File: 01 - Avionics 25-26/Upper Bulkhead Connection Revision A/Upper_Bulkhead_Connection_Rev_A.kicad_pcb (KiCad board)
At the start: 2 copper layers, 38 x 40.9 mm, 4 parts, among them J1 2601-3108, J2 M12A-08PMMP-SF8001

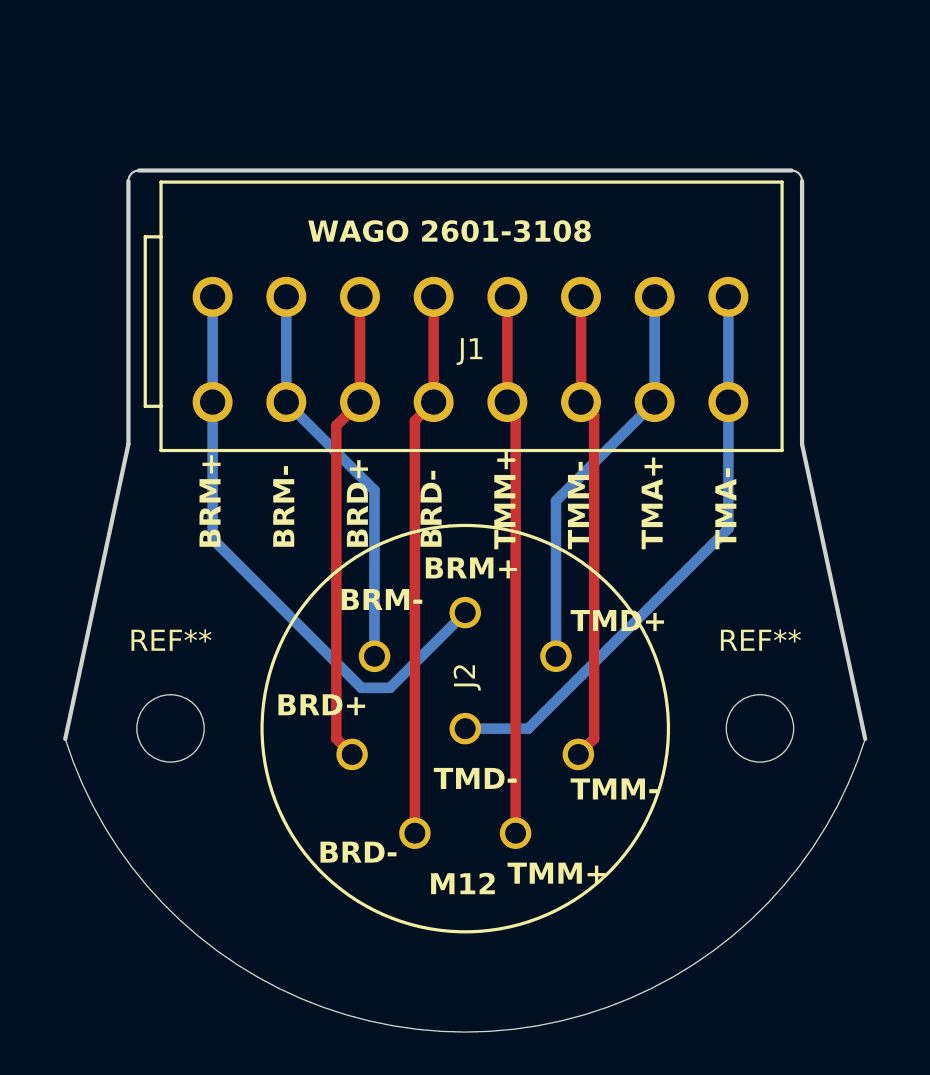
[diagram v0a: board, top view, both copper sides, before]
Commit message: Add files via upload
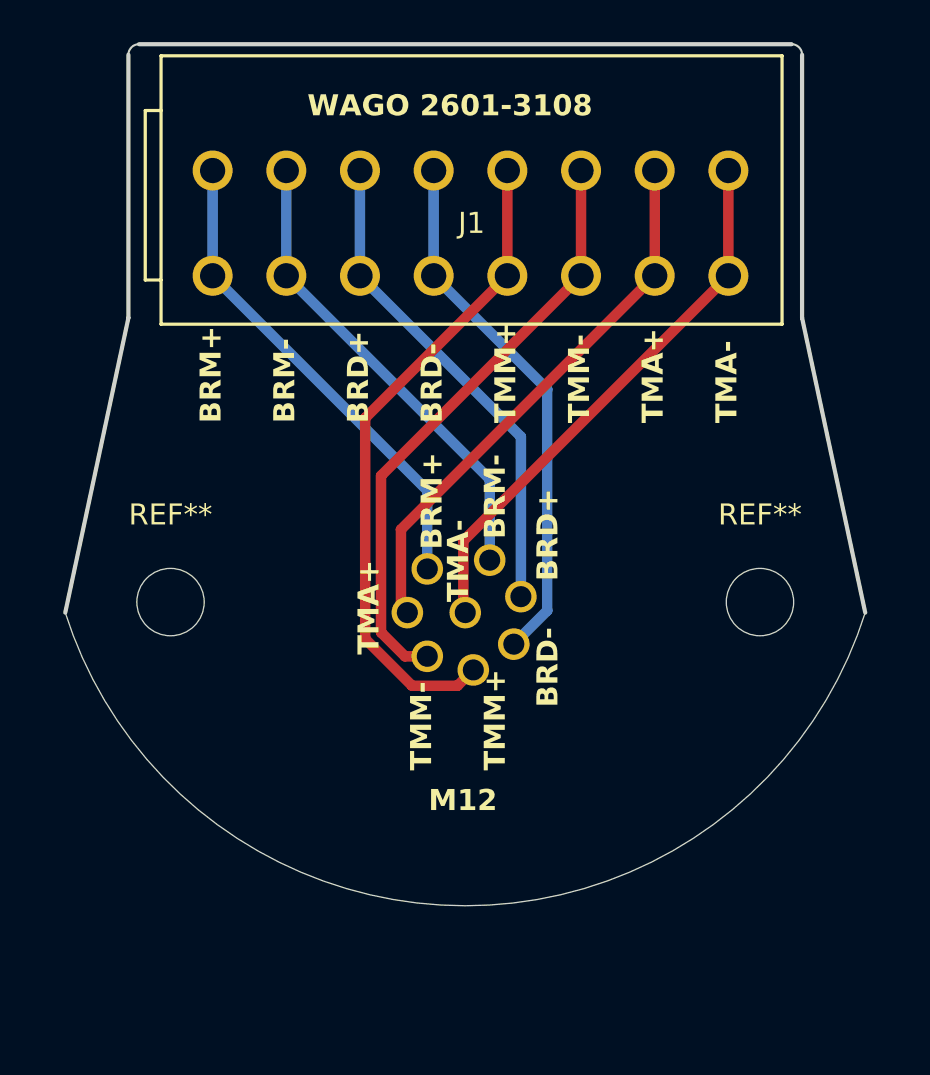
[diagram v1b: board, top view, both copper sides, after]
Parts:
- J2: moved to B.Cu
- moved J1 6.00 mm to (88.0, 79.0)
- moved REF** 6.00 mm to (86.0, 99.5)
- moved REF** 6.00 mm to (114.0, 99.5)
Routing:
- net Net-(J1-7_1): track 19.0 -> 26.1 mm
- net Net-(J1-6_1): track 22.3 -> 28.5 mm
- net Net-(J1-5_1): track 25.6 -> 31.4 mm
- net Net-(J1-1_1): track 27.9 -> 23.1 mm
- net Net-(J1-2_1): track 18.8 -> 22.5 mm
- net Net-(J1-8_1): track 27.4 -> 26.3 mm
- net Net-(J1-3_1): track 22.5 -> 23.4 mm
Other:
- board text added: "${REFERENCE}"
- board text removed: "TMD+"
- board text removed: "TMD-"

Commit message: Add files via upload
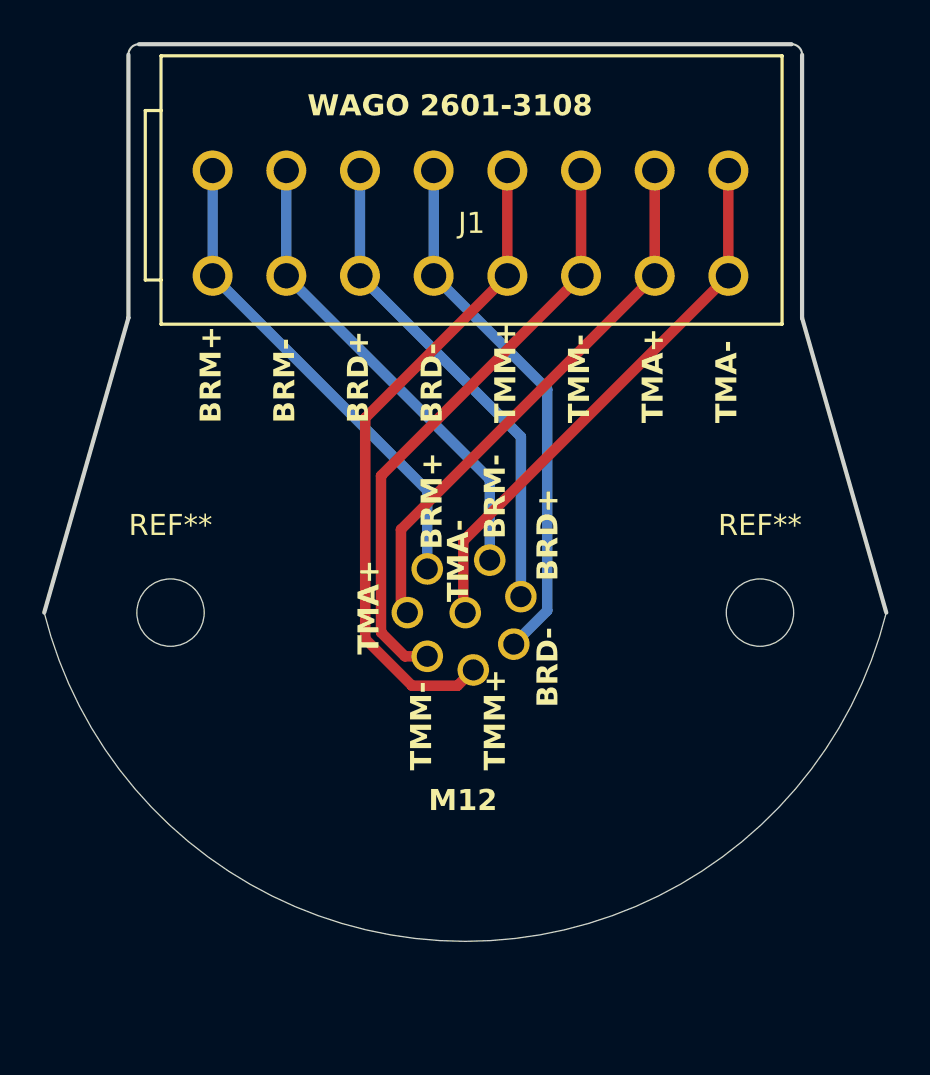
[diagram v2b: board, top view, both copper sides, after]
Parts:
- moved REF** 0.50 mm to (86.0, 100.0)
- moved REF** 0.50 mm to (114.0, 100.0)
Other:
- board size 38 x 40.9 mm -> 40 x 42.6 mm
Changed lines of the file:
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@@
 	(footprint "MountingHole:MountingHole_3.2mm_M3"
 		(layer "F.Cu")
-		(at 86 99.5)
+		(at 86 100)
 		(descr "Mounting Hole 3.2mm, M3, no annular, generated by kicad-footprint-generator mountinghole.py")
 		(tags "mountinghole M3")
@@
 	(footprint "MountingHole:MountingHole_3.2mm_M3"
 		(layer "F.Cu")
-		(at 114 99.5)
+		(at 114 100)
 		(descr "Mounting Hole 3.2mm, M3, no annular, generated by kicad-footprint-generator mountinghole.py")
 		(tags "mountinghole M3")
@@
 	(gr_line
 		(start 84 86)
-		(end 81 100)
+		(end 80 100)
 		(stroke
 			(width 0.2)
@@
 	)
 	(gr_arc
-		(start 119 100)
-		(mid 100 113.924859)
-		(end 81 100.000001)
+		(start 119.999999 100.000001)
+		(mid 100 115.615527)
+		(end 80.000001 100)
 		(stroke
 			(width 0.05)
-			(type default)
+			(type solid)
 		)
 		(layer "Edge.Cuts")
@@
 	)
 	(gr_line
-		(start 119 100)
+		(start 120 100)
 		(end 116 86)
 		(stroke
@@
 	)
 	(gr_text "${REFERENCE}"
-		(at 86 99.5 0)
+		(at 100.300001 81.5 0)
 		(layer "F.Fab")
 		(effects
@@
 	)
 	(gr_text "${REFERENCE}"
-		(at 100.300001 81.5 0)
+		(at 86 99.5 0)
 		(layer "F.Fab")
 		(effects
